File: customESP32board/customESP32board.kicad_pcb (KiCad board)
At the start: 2 copper layers, 60 x 60 mm, 43 parts, among them J1 USB_B_Micro, J2 Conn_01x16_Pin, J3 Conn_01x16_Pin, Q1 S8050, Q2 S8050, Q3 BSS138, Q4 BSS138, Q5 BSS138, U1 ESP32-WROOM-32, U2 CH340C, U3 AMS1117-3.3

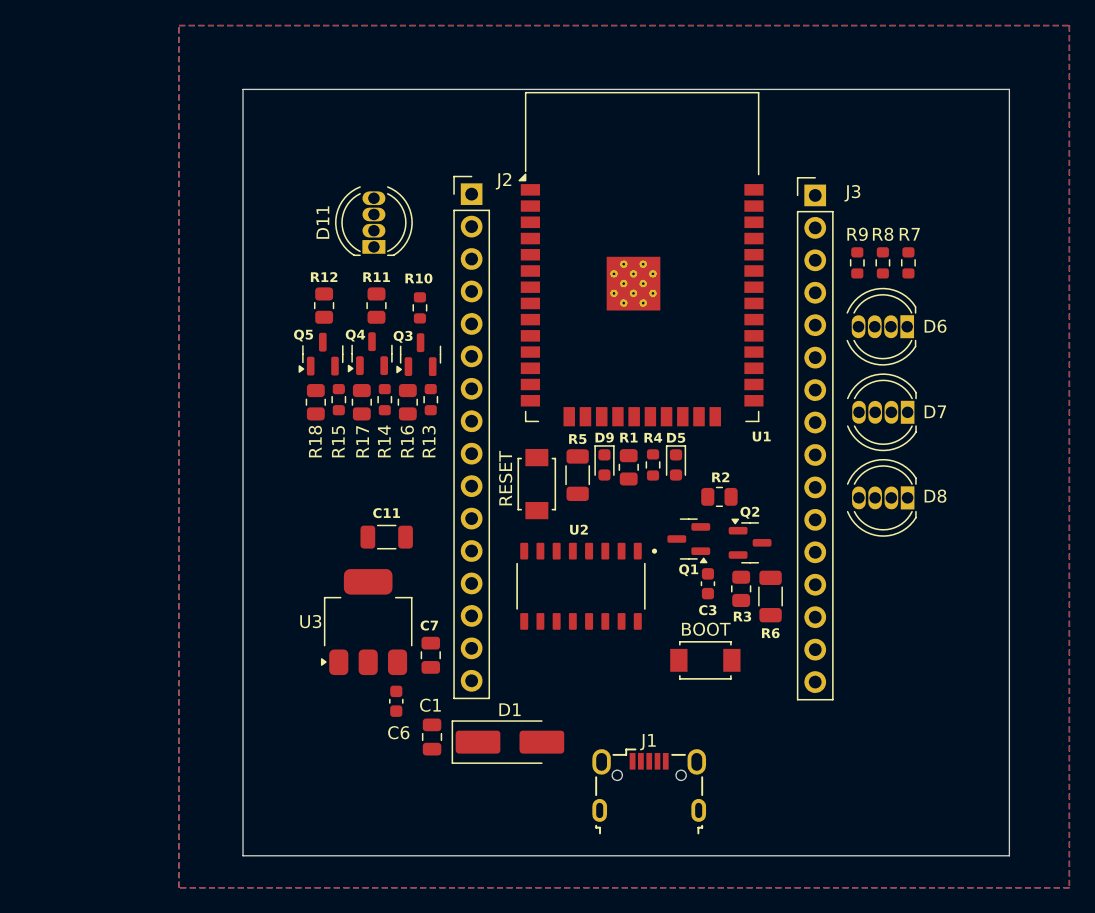
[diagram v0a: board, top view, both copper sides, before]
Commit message: finished routing
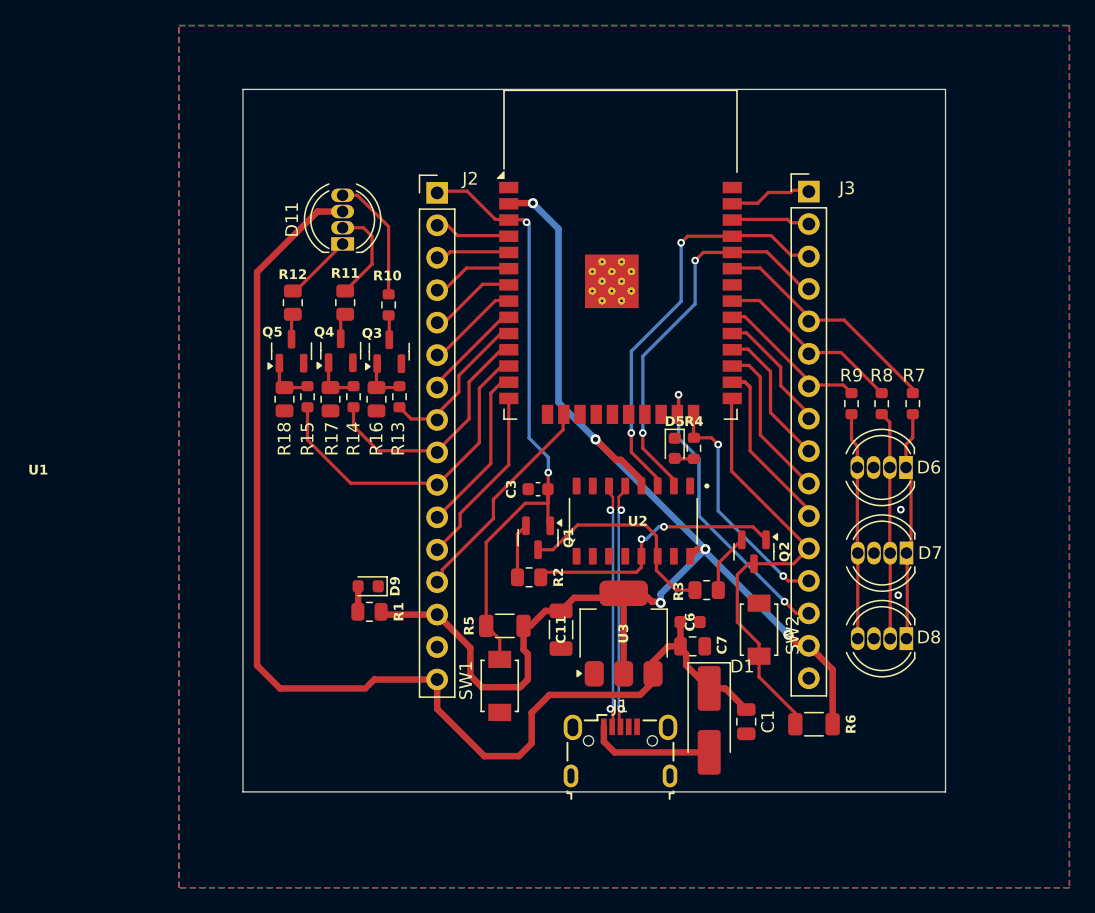
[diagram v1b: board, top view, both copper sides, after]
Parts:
- removed BOOT, RESET: SW_Push, TS-1088-AR02016:SW_TS-1088-AR02016
- added SW1: SW_Push, TS-1088-AR02016:SW_TS-1088-AR02016, F.Cu at (124.6, 120.2)
- added SW2: SW_Push, TS-1088-AR02016:SW_TS-1088-AR02016, F.Cu at (144.9, 115.8)
- moved C1 24.6 mm to (143.9, 123.0), turned to 90 degrees
- moved C6 23.8 mm to (139.5, 115.2), turned to 0 degrees
- moved R1 23.2 mm to (114.4, 114.4), turned to 0 degrees
- moved D9 20.8 mm to (114.3, 112.4), turned to 180 degrees
- moved C7 20.5 mm to (139.7, 117.1), turned to 0 degrees
- moved U3 20.0 mm to (134.3, 116.1)
- moved R2 16.2 mm to (126.9, 111.7)
- moved D1 15.7 mm to (141.0, 122.9), turned to -90 degrees
- moved C11 15.5 mm to (129.4, 115.8), turned to -90 degrees
- moved C3 15.2 mm to (127.6, 104.8), turned to 180 degrees
- moved R5 13.1 mm to (125.0, 115.5), turned to 0 degrees
- moved Q1 11.8 mm to (127.6, 108.6), turned to -90 degrees
- moved R9 11.0 mm to (152.1, 98.1)
- moved R7 11.0 mm to (156.9, 98.1)
- moved D6 11.0 mm to (156.4, 103.1)
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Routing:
- net +3V3: track 0.00 -> 104.7 mm, vias 0 -> 5
- net +5V: track 0.00 -> 92.9 mm
- net ESP_EN: track 0.00 -> 49.4 mm, vias 0 -> 2
- net ESP_IO0: track 0.00 -> 35.1 mm
- net ESP_U0TX: track 0.00 -> 32.7 mm, vias 0 -> 2
- net ESP_U0RX: track 0.00 -> 30.8 mm, vias 0 -> 2
- net ESP_IO27: track 0.00 -> 26.8 mm
- net ESP_IO15: track 0.00 -> 23.6 mm, vias 0 -> 2
- net DTR: track 0.00 -> 21.0 mm, vias 0 -> 2
- net ESP_IO26: track 0.00 -> 19.5 mm
- net UD-: track 0.00 -> 18.9 mm, vias 0 -> 2
- net ESP_IO21: track 0.00 -> 18.8 mm
- net ESP_IO2: track 0.00 -> 18.7 mm, vias 0 -> 2
- net UD+: track 0.00 -> 18.5 mm, vias 0 -> 2
- net RGB_BLUE: track 0.00 -> 18.2 mm
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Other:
- board size 60 x 60 mm -> 55 x 55 mm
